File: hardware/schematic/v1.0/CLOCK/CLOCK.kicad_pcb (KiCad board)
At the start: 2 copper layers, 90 x 90 mm, 131 parts, among them J1 Conn_Coaxial, J10 Conn_Coaxial, J12 Conn_Coaxial, J14 Conn_01x16_Socket, J2 Conn_Coaxial, J3 Conn_Coaxial, J4 Conn_Coaxial, J5 Conn_Coaxial, J6 Conn_Coaxial, J7 Conn_Coaxial, J8 Conn_Coaxial, J9 Conn_Coaxial, U1 LMK5B12204, U2 LMK1C1102, U3 LMK1C1102, U4 TPS78633, U5 TPS78633, U6 OCXO-10M, U7 TPS63020DSJR

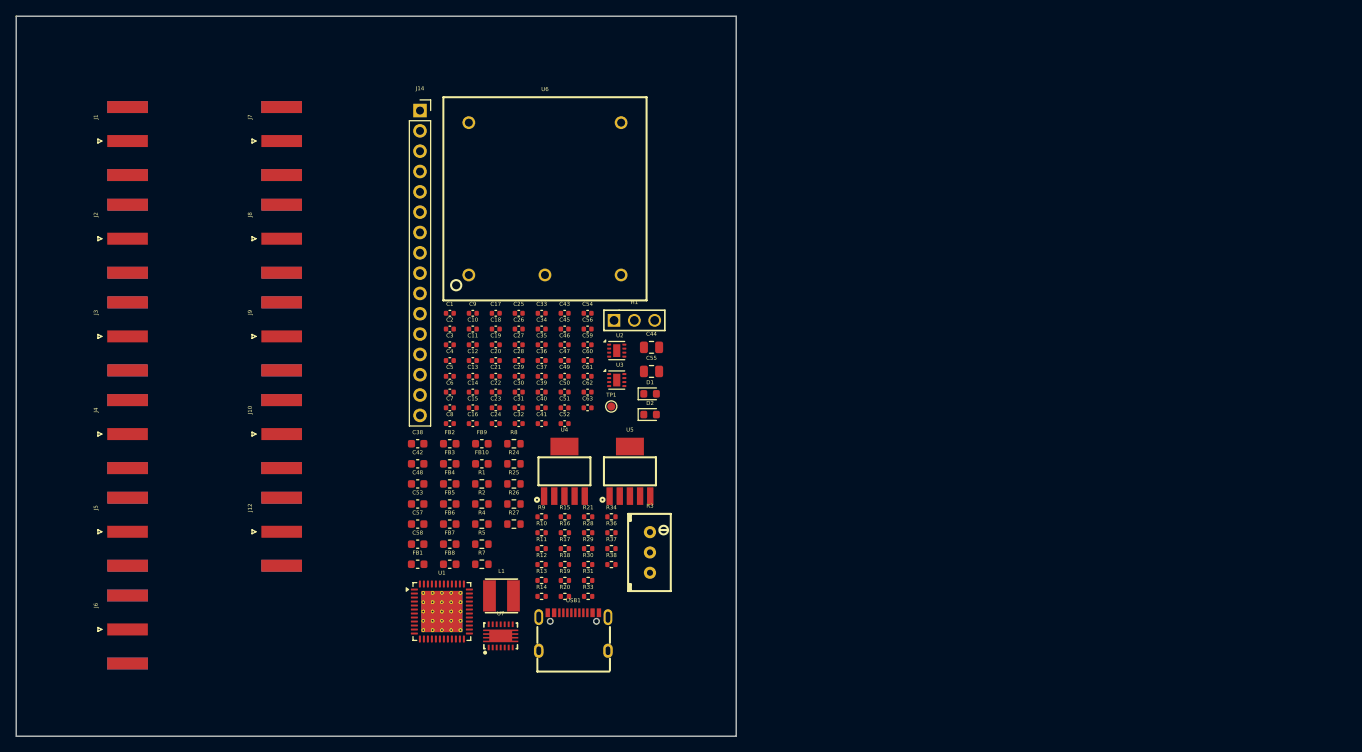
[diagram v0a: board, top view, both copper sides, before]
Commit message: pcb update
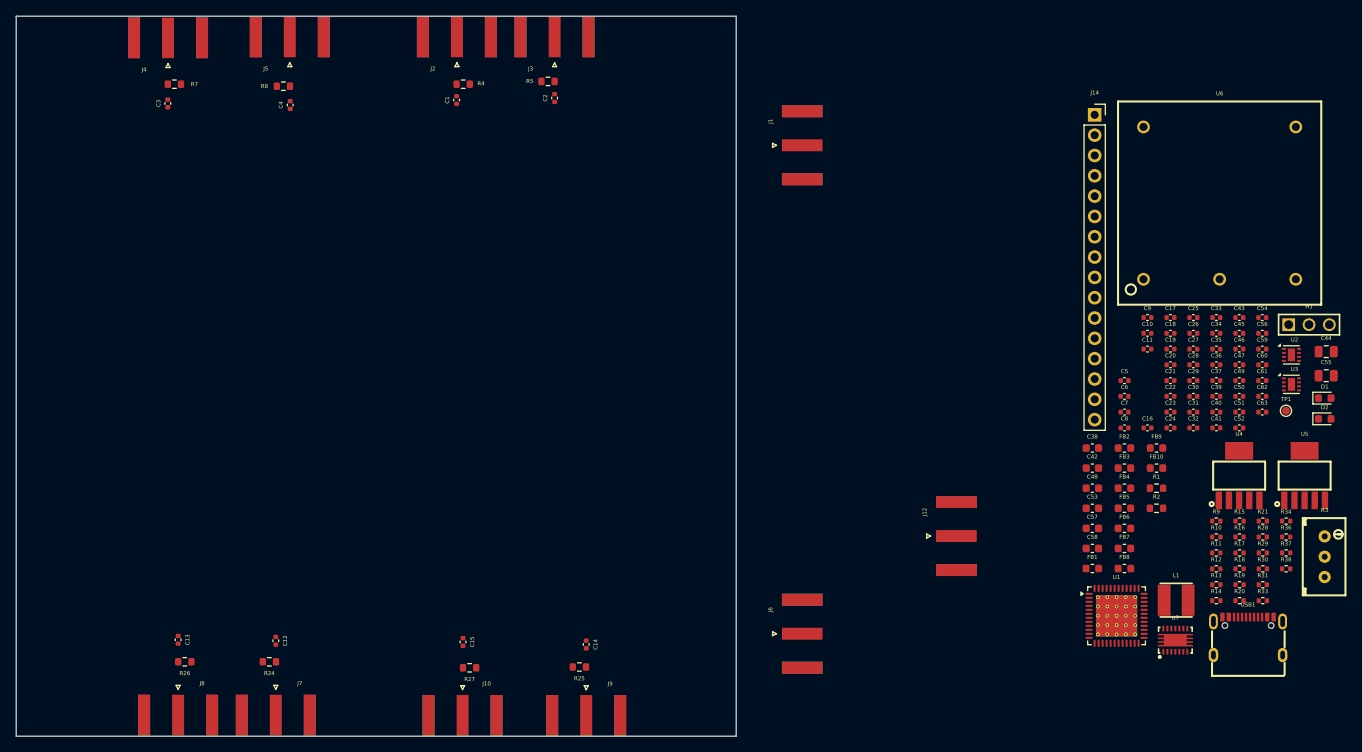
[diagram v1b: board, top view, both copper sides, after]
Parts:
- moved C10 84.3 mm to (237.2, 92.5)
- moved C11 84.3 mm to (237.2, 94.5)
- moved C16 84.3 mm to (237.2, 104.3)
- moved C17 84.3 mm to (240.0, 90.5)
- moved C18 84.3 mm to (240.0, 92.5)
- moved C19 84.3 mm to (240.0, 94.5)
- moved C20 84.3 mm to (240.0, 96.4)
- moved C21 84.3 mm to (240.0, 98.4)
- moved C22 84.3 mm to (240.0, 100.4)
- moved C23 84.3 mm to (240.0, 102.3)
- moved C24 84.3 mm to (240.0, 104.3)
- moved C25 84.3 mm to (242.9, 90.5)
- moved C26 84.3 mm to (242.9, 92.5)
- moved C27 84.3 mm to (242.9, 94.5)
- moved C28 84.3 mm to (242.9, 96.4)
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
